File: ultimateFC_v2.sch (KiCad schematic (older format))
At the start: 196 parts, among them J1 USB_B_Micro, J2 10132797-011100LF, J3 10132797-011100LF, J4 10132797-011100LF, J5 10132797-011100LF, J6 10132797-011100LF, Q1 DMP2066LSN-7, U1 EFM8BB21F16G-C-QFN20R, U10 NCP81253MNTBG, U11 SiZ200DT, U12 NCP81253MNTBG, U13 SiZ200DT, U14 TPS62821, U15 SiZ200DT, U16 NCP81253MNTBG, U17 NCP81253MNTBG, U18 NCP81253MNTBG, U19 NCP81253MNTBG, U2 EFM8BB21F16G-C-QFN20R, U20 SiZ200DT, U21 SiZ200DT, U22 SiZ200DT, U23 SiZ200DT, U24 EFM8BB21F16G-C-QFN20R, U25 NCP81253MNTBG, U26 SiZ200DT, U27 NCP81253MNTBG, U28 NCP81253MNTBG, U29 SiZ200DT, U3 NCP81253MNTBG, U30 SiZ200DT, U31 INA186, U32 LMR33630CQRNX, U33 STM32F745VGHx, U34 AB7456, U35 ZOE-M8Q_ZOE-M8Q, U36 ICM-20602, U37 S25FL064L, U38 LIS3MDL, U39 BMP280, U4 SiZ200DT, U5 TPS630701, U6 EFM8BB21F16G-C-QFN20R, U7 NCP81253MNTBG, U8 SiZ200DT, U9 NCP81253MNTBG, X1 Molex_734120110, Y1 CSTNE8M00G550000R0, Y2 ECS-270-8-47Q-CES-TR

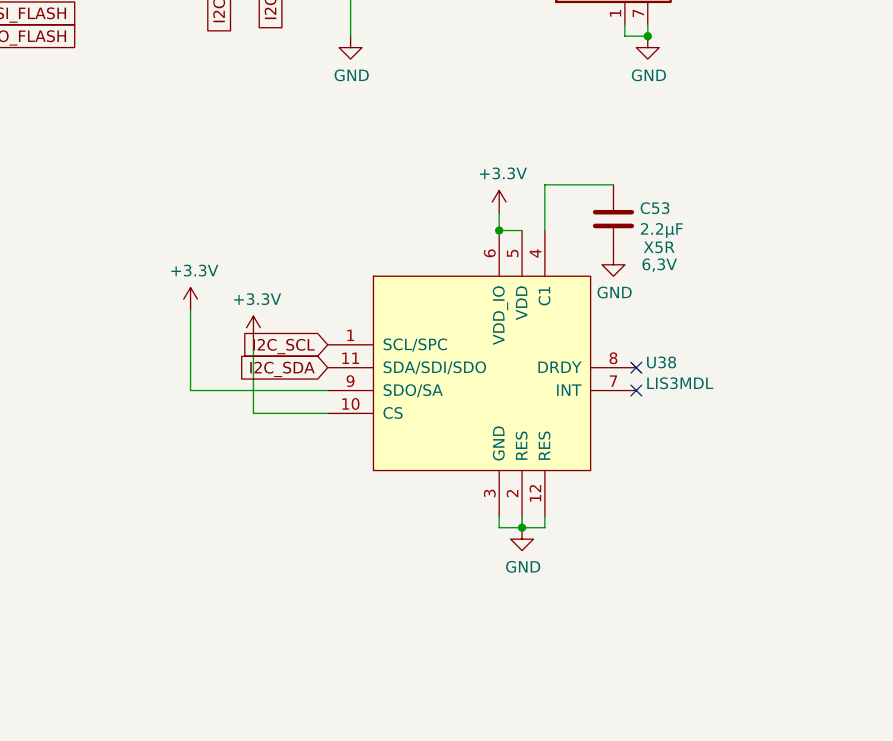
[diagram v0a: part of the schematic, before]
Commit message: update layout
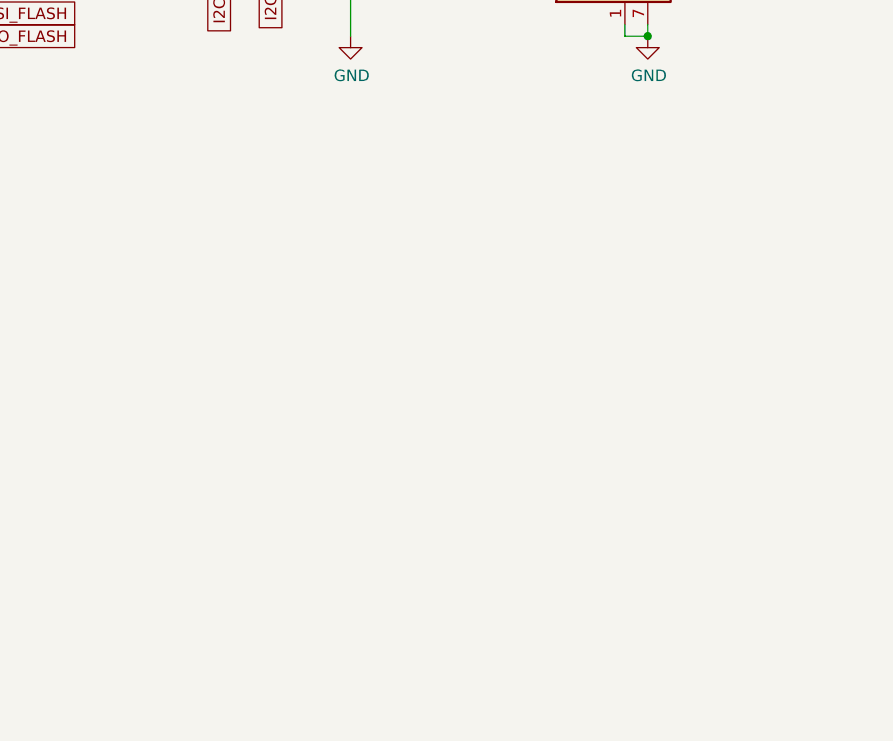
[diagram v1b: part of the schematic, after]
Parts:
- removed C53: 2.2µF, Capacitor_SMD:C_0402_1005Metric, symbol Device:C
- removed U38: LIS3MDL, Package_LGA:LGA-12_2x2mm_P0.5mm, symbol own_devices:LIS3MDL
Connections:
- no-connect marks 43 -> 41
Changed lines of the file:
@@
 EESchema Schematic File Version 4
-LIBS:ultimateFC-cache
 EELAYER 30 0
 EELAYER END
@@
 	1    0    0    -1
 $EndComp
-$Comp
-L Device:C C53
-U 1 1 60374537
-P 30100 9225
-F 0 "C53" H 30215 9271 50  0000 L CNN
-F 1 "2.2µF" H 30215 9180 50  0000 L CNN
-F 2 "Capacitor_SMD:C_0402_1005Metric" H 30138 9075 50  0001 C CNN
-F 3 "~" H 30100 9225 50  0001 C CNN
-F 4 "6,3V" H 30300 9025 50  0000 C CNN "Spannung"
-F 5 "X5R" H 30300 9100 50  0000 C CNN "Dielektrikum"
-F 6 "C0402C225M9PACTU" H 30100 9225 50  0001 C CNN "Mfr.No:"
-F 7 "0,093" H 30100 9225 50  0001 C CNN "price@100[€]"
-F 8 "0,08" H 30100 9225 50  0001 C CNN "price@10[€]"
-F 9 "0,043" H 30100 9225 50  0001 C CNN "price@1k[€]"
-	1    30100 9225
-	1    0    0    -1
-$EndComp
 Wire Wire Line
 	28950 8075 29750 8075
@@
 	28950 8075 28950 8425
 Wire Wire Line
-	28250 9975 28850 9975
-Wire Wire Line
-	28250 9625 28250 9975
-Wire Wire Line
 	29250 8175 29750 8175
 Wire Wire Line
@@
 	1    0    0    -1
 $EndComp
-$Comp
-L power:+3.3V #PWR0190
-U 1 1 5D2A0549
-P 28250 9625
-F 0 "#PWR0190" H 28250 9475 50  0001 C CNN
-F 1 "+3.3V" H 28265 9798 50  0000 C CNN
-F 2 "" H 28250 9625 50  0001 C CNN
-F 3 "" H 28250 9625 50  0001 C CNN
-	1    28250 9625
-	1    0    0    -1
-$EndComp
-Wire Wire Line
-	28525 10075 28850 10075
-Wire Wire Line
-	28525 9750 28525 10075
-$Comp
-L power:+3.3V #PWR0191
-U 1 1 5D29BED3
-P 28525 9750
-F 0 "#PWR0191" H 28525 9600 50  0001 C CNN
-F 1 "+3.3V" H 28540 9923 50  0000 C CNN
-F 2 "" H 28525 9750 50  0001 C CNN
-F 3 "" H 28525 9750 50  0001 C CNN
-	1    28525 9750
-	1    0    0    -1
-$EndComp
-Wire Wire Line
-	29800 9075 30100 9075
-Wire Wire Line
-	29800 9275 29800 9075
-$Comp
-L power:GND #PWR0313
-U 1 1 5D278DB0
-P 30100 9375
-F 0 "#PWR0313" H 30100 9125 50  0001 C CNN
-F 1 "GND" H 30105 9202 50  0000 C CNN
-F 2 "" H 30100 9375 50  0001 C CNN
-F 3 "" H 30100 9375 50  0001 C CNN
-	1    30100 9375
-	1    0    0    -1
-$EndComp
 Wire Wire Line
 	30250 7650 30250 7675
@@
 	1    0    0    -1
 $EndComp
-NoConn ~ 30200 9975
-NoConn ~ 30200 9875
-Connection ~ 29600 9275
-Wire Wire Line
-	29700 9275 29600 9275
-Wire Wire Line
-	29600 9200 29600 9275
-$Comp
-L power:+3.3V #PWR0320
-U 1 1 5D277896
-P 29600 9200
-F 0 "#PWR0320" H 29600 9050 50  0001 C CNN
-F 1 "+3.3V" H 29615 9373 50  0000 C CNN
-F 2 "" H 29600 9200 50  0001 C CNN
-F 3 "" H 29600 9200 50  0001 C CNN
-	1    29600 9200
-	1    0    0    -1
-$EndComp
-Wire Wire Line
-	29700 10525 29700 10575
-Wire Wire Line
-	29700 10575 29800 10575
-Connection ~ 29700 10575
-Wire Wire Line
-	29800 10575 29800 10525
-Wire Wire Line
-	29600 10575 29700 10575
-Wire Wire Line
-	29600 10525 29600 10575
-$Comp
-L power:GND #PWR0321
-U 1 1 5D277823
-P 29700 10575
-F 0 "#PWR0321" H 29700 10325 50  0001 C CNN
-F 1 "GND" H 29705 10402 50  0000 C CNN
-F 2 "" H 29700 10575 50  0001 C CNN
-F 3 "" H 29700 10575 50  0001 C CNN
-	1    29700 10575
-	1    0    0    -1
-$EndComp
-$Comp
-L own_devices:LIS3MDL U38
-U 1 1 5D2776BA
-P 29600 9925
-F 0 "U38" H 30241 9996 50  0000 L CNN
-F 1 "LIS3MDL" H 30241 9905 50  0000 L CNN
-F 2 "Package_LGA:LGA-12_2x2mm_P0.5mm" H 29450 10025 50  0001 C CNN
-F 3 "" H 29450 10025 50  0001 C CNN
-	1    29600 9925
-	1    0    0    -1
-$EndComp
 $Comp
 L Sensor_Pressure:BMP280 U39
@@
 Text GLabel 29625 7975 0    50   Input ~ 0
 I2C_SDA
-Text GLabel 28850 9775 0    50   Input ~ 0
-I2C_SCL
-Text GLabel 28850 9875 0    50   Input ~ 0
-I2C_SDA
 $Comp

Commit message: update schematic
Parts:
- C1, C2: footprint Capacitor_SMD:C_1206_3216Metric -> Capacitor_SMD:C_0805_2012Metric
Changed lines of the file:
@@
 F 0 "C2" H 2240 12221 50  0000 L CNN
 F 1 "10µF" H 2240 12130 50  0000 L CNN
-F 2 "Capacitor_SMD:C_1206_3216Metric" H 2163 12025 50  0001 C CNN
+F 2 "Capacitor_SMD:C_0805_2012Metric" H 2163 12025 50  0001 C CNN
 F 3 "~" H 2125 12175 50  0001 C CNN
 F 4 "25V" H 2325 11975 50  0000 C CNN "Spannung"
@@
 F 0 "C1" H 1815 12221 50  0000 L CNN
 F 1 "10µF" H 1815 12130 50  0000 L CNN
-F 2 "Capacitor_SMD:C_1206_3216Metric" H 1738 12025 50  0001 C CNN
+F 2 "Capacitor_SMD:C_0805_2012Metric" H 1738 12025 50  0001 C CNN
 F 3 "~" H 1700 12175 50  0001 C CNN
 F 4 "25V" H 1900 11975 50  0000 C CNN "Spannung"
